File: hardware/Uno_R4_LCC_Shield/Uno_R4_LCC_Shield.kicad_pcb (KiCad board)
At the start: 2 copper layers, 68.8 x 53.6 mm, 33 parts, among them J1 A00-216-262-450, J2 54-00166, J3 Screw_Terminal_01x02, SW1 SW_Push, U1 ACPL-214-500E, U2 7410, U3 7410, U4 7410, U5 7410, U6 DRV8874PWPR, U7 MCP2562-E-SN

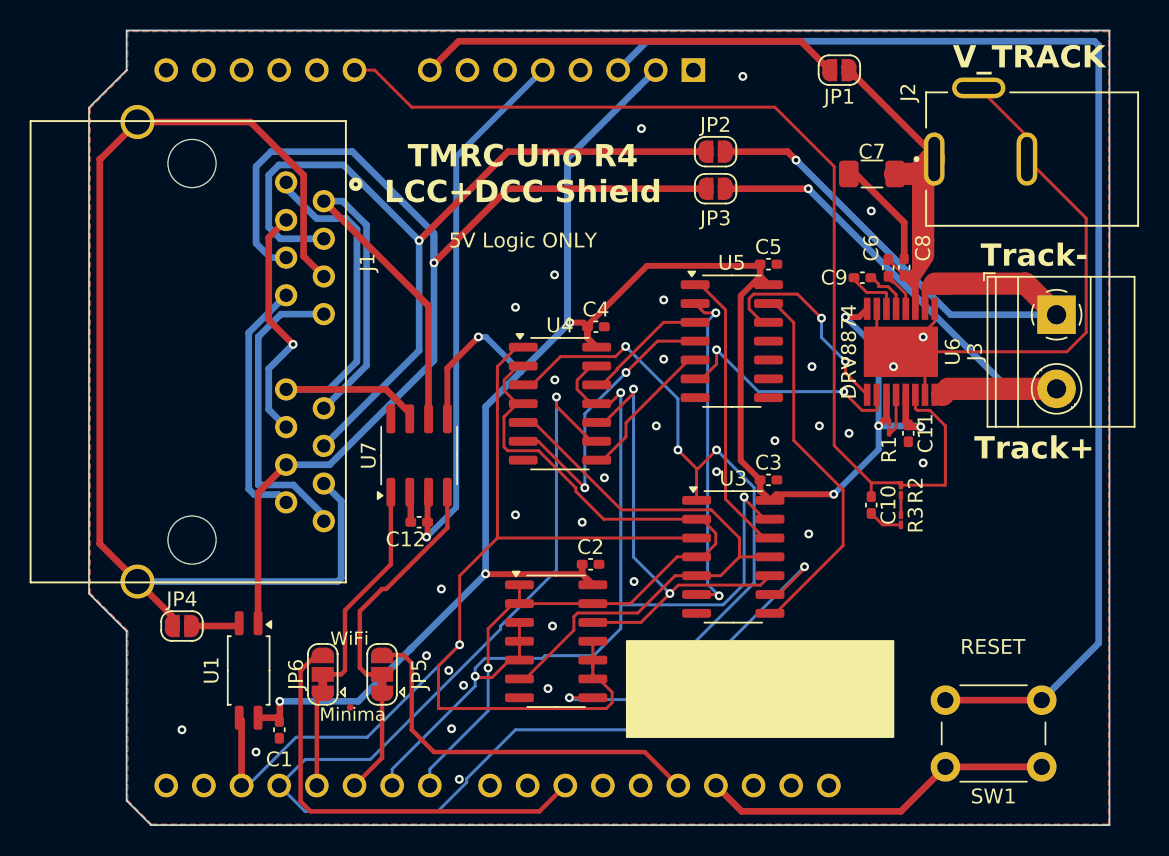
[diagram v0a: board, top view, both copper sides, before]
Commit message: Update to hardware v2 and cleanup
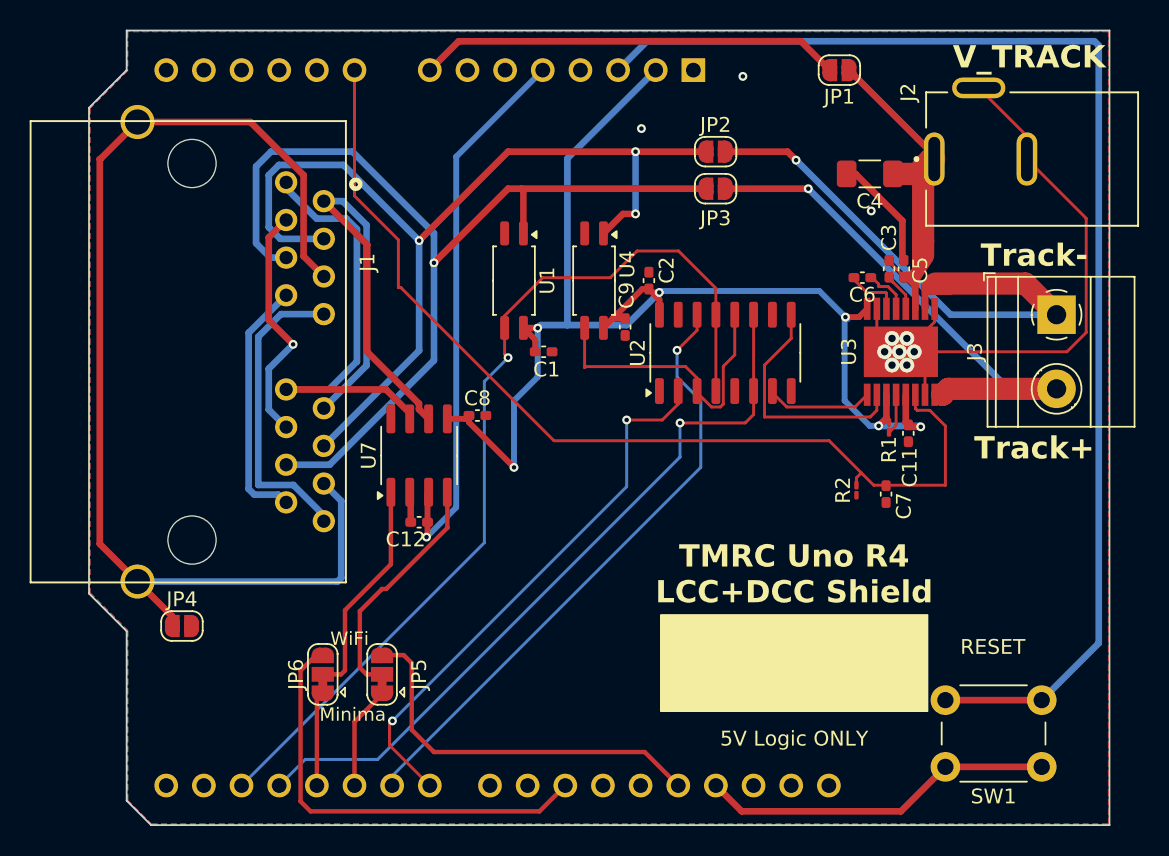
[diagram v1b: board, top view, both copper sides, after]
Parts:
- removed C10: C22n, Capacitor_SMD:C_0402_1005Metric_Pad0.74x0.62mm_HandSolder
- removed R3: R732, Resistor_SMD:R_01005_0402Metric_Pad0.57x0.30mm_HandSolder
- removed U5: 7410, Package_SO:SOIC-14_3.9x8.7mm_P1.27mm
- removed U6: DRV8874PWPR, ul_DRV8874PWPR:PWP0016J_NV
- C4: value C100n -> C10u; footprint Capacitor_SMD:C_0402_1005Metric_Pad0.74x0.62mm_HandSolder -> Capacitor_SMD:C_1206_3216Metric_Pad1.33x1.80mm_HandSolder
- C6: value C100n -> C22n
- C7: value C10u -> C22n; footprint Capacitor_SMD:C_1206_3216Metric_Pad1.33x1.80mm_HandSolder -> Capacitor_SMD:C_0402_1005Metric_Pad0.74x0.62mm_HandSolder
- C9: value C22n -> C100n
- R2: value R1k43 -> R2k
- U2: value 7410 -> SN74HC253DR; footprint Package_SO:SOIC-14_3.9x8.7mm_P1.27mm -> Package_SO:SO-16_3.9x9.9mm_P1.27mm
- U3: value 7410 -> DRV8874PWPR; footprint Package_SO:SOIC-14_3.9x8.7mm_P1.27mm -> DRV8874PWPR:PWP0016J_NV
- U4: value 7410 -> ACPL-214-500E; footprint Package_SO:SOIC-14_3.9x8.7mm_P1.27mm -> Package_SO:SOP-4_4.4x2.6mm_P1.27mm
- moved U1 31.8 mm to (125.4, 38.2)
- moved C1 31.1 mm to (127.4, 43.0), turned to 0 degrees
- moved C8 30.5 mm to (122.9, 47.3), turned to 0 degrees
- moved U2 22.6 mm to (139.7, 43.1), turned to 90 degrees
- moved C7 21.6 mm to (150.5, 52.6), turned to -90 degrees
- moved C4 21.2 mm to (149.4, 31.0), turned to 180 degrees
- moved C2 19.5 mm to (134.5, 38.2), turned to 90 degrees
- moved U3 17.9 mm to (151.5, 43.0), turned to 90 degrees
- moved C3 16.4 mm to (150.7, 37.4), turned to -90 degrees
- moved C9 16.3 mm to (132.9, 41.3), turned to -90 degrees
- moved C5 9.14 mm to (151.7, 37.4), turned to 90 degrees
- moved U4 8.61 mm to (130.8, 38.2), turned to -90 degrees
- moved R2 3.00 mm to (148.5, 52.3)
- moved C6 1.86 mm to (148.9, 38.0), turned to 180 degrees
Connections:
- C3 pad 1: IOREF -> VTRACK
- C3 pad 2: GND -> Net-(U3-VCP)
- C4 pad 1: IOREF -> VTRACK
- C5 pad 1: IOREF -> VTRACK
- C6 pad 1: VTRACK -> Net-(U3-CPH)
- C6 pad 2: Net-(U6-VCP) -> Net-(U3-CPL)
- C7 pad 1: VTRACK -> /sense_A
- C8 pad 1: VTRACK -> IOREF
- C9 pad 1: Net-(U6-CPH) -> IOREF
- C9 pad 2: Net-(U6-CPL) -> GND
- R1 pad 2: Net-(U6-FAULT_N) -> Net-(U3-FAULT_N)
- R2 pad 2: Net-(R2-Pad2) -> GND
- U2 pad 1: /dcc_en_A -> GND
- U2 pad 10: /dcc_p -> GND
- U2 pad 11: /dcc_p -> /pwm_A
- U2 pad 12: Net-(U2-Pad12) -> /dcc_n
- U2 pad 13: /dcc_en_A -> /dcc_p
- U2 pad 14: IOREF -> /dir_A
- U2 pad 3: /dir_A -> /dcc_n
- U2 pad 4: /dir_A -> /dcc_p
- U2 pad 5: /dir_A -> GND
- U2 pad 6: Net-(U2-Pad6) -> /pwm_A
- U2 pad 7: GND -> Net-(U2-1Y)
- U2 pad 8: Net-(U2-Pad8) -> GND
- U2 pad 9: /dcc_p -> Net-(U2-2Y)
- U3 pad 1: Net-(U2-Pad8) -> Net-(U2-1Y)
- U3 pad 10: Net-(U2-Pad12) -> /out2_A
- U3 pad 11: Net-(U2-Pad6) -> VTRACK
- U3 pad 12: Net-(U3-Pad12) -> Net-(U3-VCP)
- U3 pad 13: /dir_A -> Net-(U3-CPH)
- U3 pad 14: IOREF -> Net-(U3-CPL)
- U3 pad 2: /dcc_en_A -> Net-(U2-2Y)
- U3 pad 3: /dcc_p -> IOREF
- U3 pad 4: /dcc_en_A -> Net-(U3-FAULT_N)
- U3 pad 5: Net-(U2-Pad6) -> IOREF
- U3 pad 6: Net-(U3-Pad6) -> /sense_A
- U3 pad 8: Net-(U3-Pad8) -> /out1_A
- U3 pad 9: /pwm_A -> GND
- U4 pad 1: /dcc_p -> /raw_dcc_n
- U4 pad 2: /dcc_en_A -> GND
- U4 pad 3: Net-(U2-Pad8) -> /dcc_n
- U4 pad 4: /dcc_en_A -> IOREF
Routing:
- net IOREF: track 152.7 -> 89.9 mm, vias 8 -> 6
- net Net-(U2-Pad8): track 49.6 -> 0.00 mm, vias 4 -> 0
- net Net-(U2-Pad6): track 39.9 -> 0.00 mm
- net /pwm_A: track 87.2 -> 50.5 mm, vias 2 -> 1
- net Net-(U2-Pad12): track 31.7 -> 0.00 mm, vias 2 -> 0
- net Net-(U3-Pad8): track 25.5 -> 0.00 mm
- net /dir_A: track 66.6 -> 41.6 mm, vias 3 -> 1
- net Net-(U3-Pad6): track 23.0 -> 0.00 mm, vias 2 -> 0
- net /dcc_n: track 0.00 -> 20.2 mm
- net Net-(U4-Pad6): track 19.9 -> 0.00 mm, vias 2 -> 0
- net Net-(U3-Pad12): track 19.6 -> 0.00 mm
- net /dcc_p: track 82.3 -> 63.3 mm
- net /dcc_en_A: track 56.1 -> 37.2 mm, vias 1 -> 2
- net Net-(U2-2Y): track 0.00 -> 16.5 mm
- net Net-(U6-PH_IN2): track 16.4 -> 0.00 mm, vias 2 -> 0
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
